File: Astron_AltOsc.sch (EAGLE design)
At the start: 10 parts, among them J1 CONN_6SCREW_2.54, U1 MCP7940SOIC

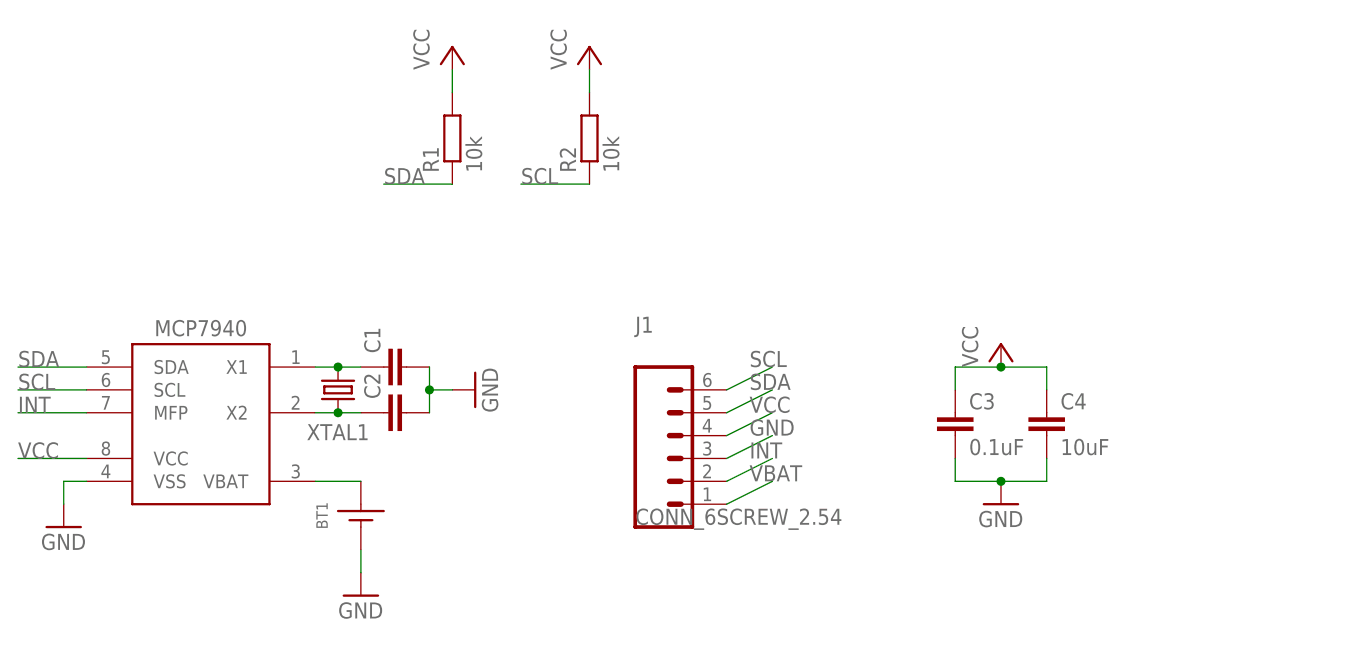
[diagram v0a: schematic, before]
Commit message: Minor updates and added gerber
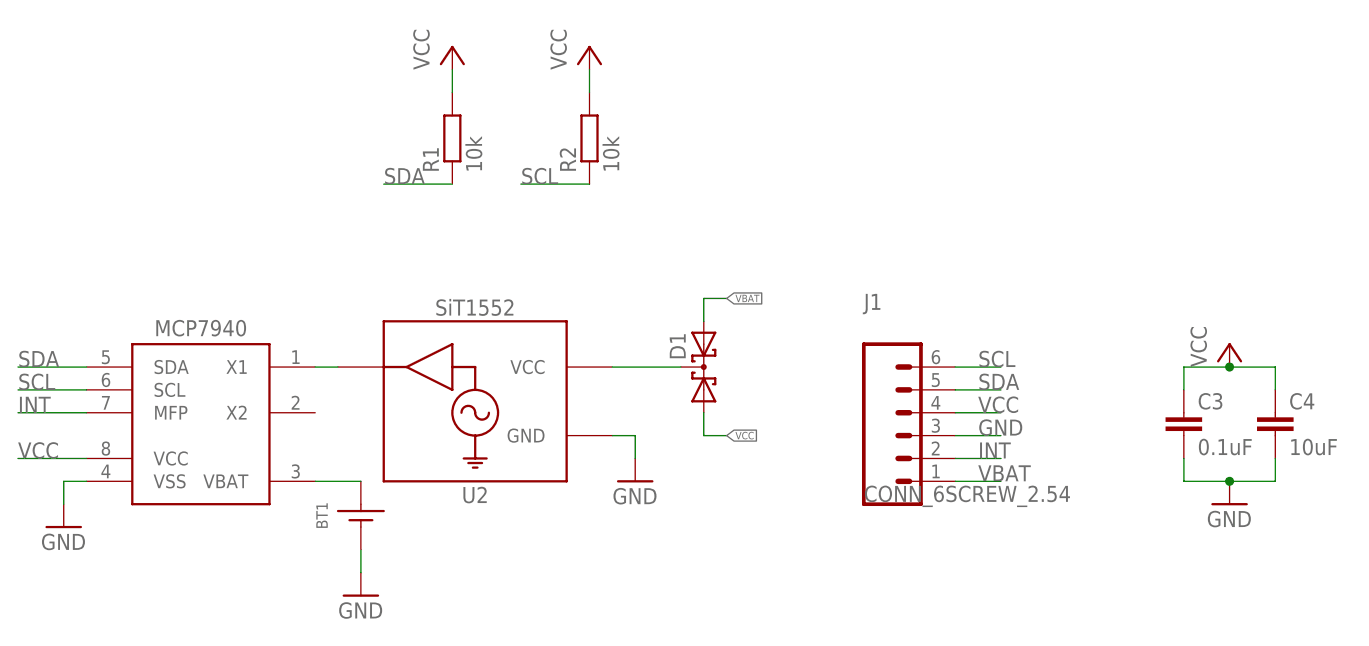
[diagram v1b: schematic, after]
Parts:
- removed C1, C2: (no value), bschulz_passives:C-EUC0603
- removed XTAL1: CRYSTAL3.2X1.5, bschulz:CRYSTAL3.2X1.5
- added D1: (no value), bschulz:DIODE_CCBAT54CSOT23
- added U2: SIT1552, bschulz:SIT1552
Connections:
- net GND: now also U2.GND; no longer C1.2, C2.2
- net N$1: now also U2.CLK; no longer C1.1, XTAL1.1
- net N$2: now also D1.C, U2.VCC; no longer C2.1, U1.X2, XTAL1.2
- net VBAT: now also D1.A2
- net VCC: now also D1.A1
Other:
- moved on the sheet: C3, C4, J1
